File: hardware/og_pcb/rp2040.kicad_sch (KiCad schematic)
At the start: 29 parts, among them J11 Conn_02x02_Top_Bottom, J4 Micro_SD_Card_Det1, SW4 SW_Push_Shielded, SW5 SW_Push_Shielded, U12 RP2040, U3 W25Q128JVS, Y3 ABM8-272-T3

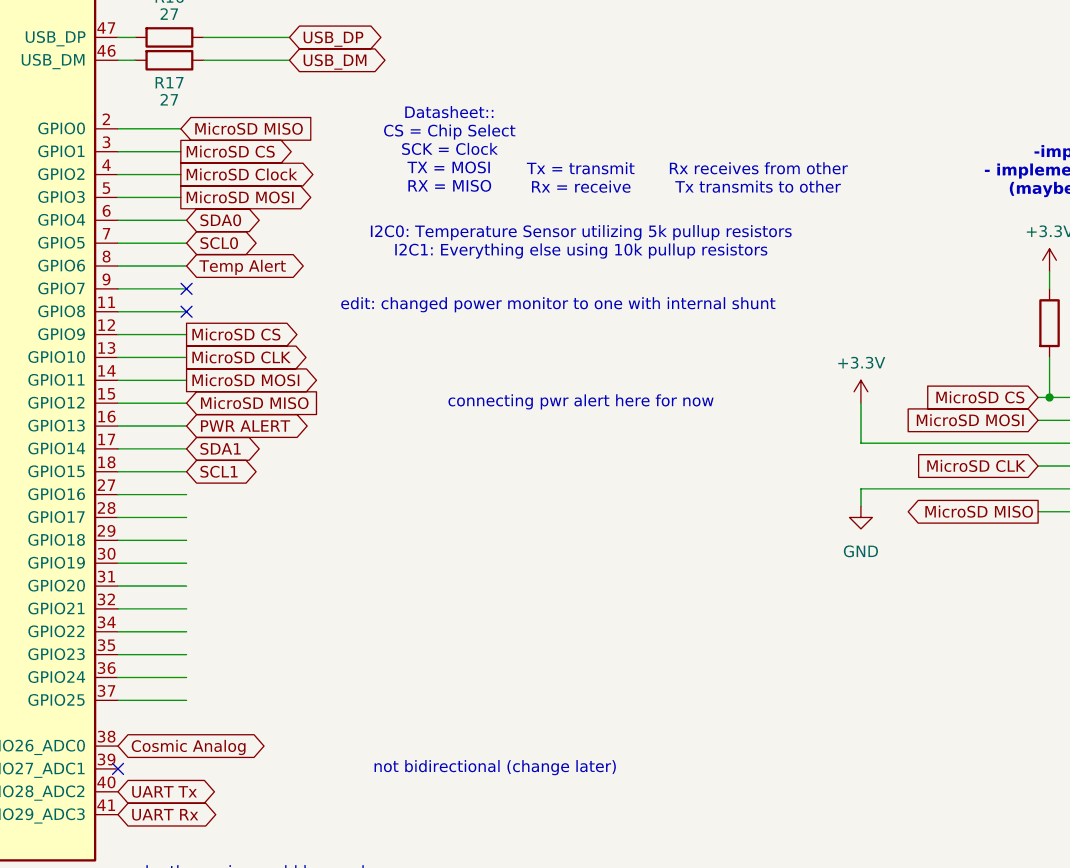
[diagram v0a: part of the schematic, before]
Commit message: new preliminary demo pcb
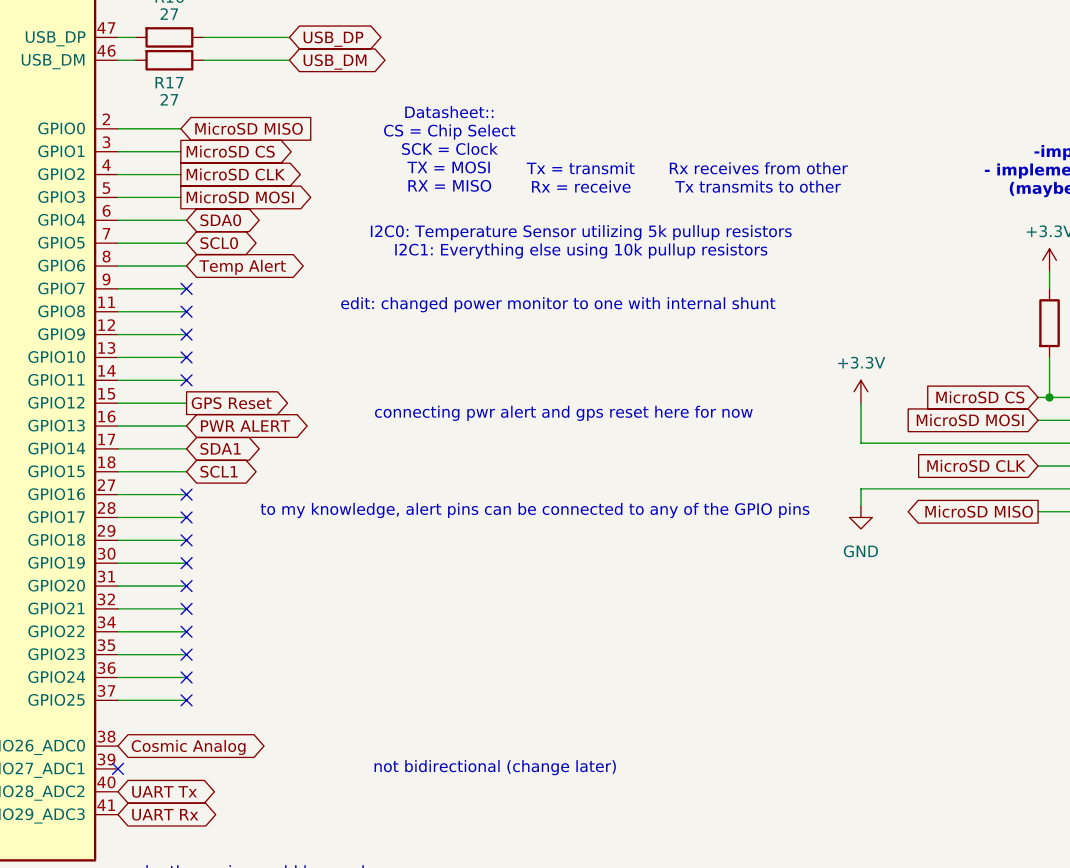
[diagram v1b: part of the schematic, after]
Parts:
- J4: footprint (none) -> 1my_footprints:microSD-503398-1892-1
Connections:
- net MicroSD Clock is gone; now on net MicroSD CLK: U12.4 (GPIO2)
- net MicroSD CLK: no longer U12.13 (GPIO10)
- net MicroSD CS: no longer U12.12 (GPIO9)
- net MicroSD MISO: no longer U12.15 (GPIO12)
- net MicroSD MOSI: no longer U12.14 (GPIO11)
- new net GPS Reset: U12.15 (GPIO12)
- no-connect marks 6 -> 19
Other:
- note added: "connecting pwr alert and gps reset here for now"
- note added: "to my knowledge, alert pins can be connected to any of the GPIO pins"
- note removed: "connecting pwr alert here for now"
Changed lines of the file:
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@@
 		)
 	)
+	(text "to my knowledge, alert pins can be connected to any of the GPIO pins"
+		(exclude_from_sim no)
+		(at 163.83 138.43 0)
+		(effects
+			(font
+				(size 1.27 1.27)
+			)
+		)
+	)
 	(text "Flash"
 		(exclude_from_sim no)
@@
 		)
 	)
-	(text "connecting pwr alert here for now"
+	(text "connecting pwr alert and gps reset here for now"
 		(exclude_from_sim no)
-		(at 168.91 126.365 0)
+		(at 167.005 127.635 0)
 		(effects
 			(font
@@
 	)
 	(no_connect
+		(at 125.095 154.305)
+	)
+	(no_connect
 		(at 227.33 146.05)
 	)
 	(no_connect
+		(at 125.095 149.225)
+	)
+	(no_connect
+		(at 125.095 159.385)
+	)
+	(no_connect
 		(at 125.095 116.205)
 	)
 	(no_connect
+		(at 125.095 146.685)
+	)
+	(no_connect
 		(at 125.095 113.665)
 	)
@@
 	)
 	(no_connect
+		(at 125.095 136.525)
+	)
+	(no_connect
+		(at 125.095 139.065)
+	)
+	(no_connect
+		(at 125.095 123.825)
+	)
+	(no_connect
 		(at 227.33 140.97)
 	)
 	(no_connect
+		(at 125.095 118.745)
+	)
+	(no_connect
+		(at 125.095 144.145)
+	)
+	(no_connect
+		(at 125.095 121.285)
+	)
+	(no_connect
+		(at 125.095 151.765)
+	)
+	(no_connect
 		(at 227.33 123.19)
 	)
+	(no_connect
+		(at 125.095 156.845)
+	)
+	(no_connect
+		(at 125.095 141.605)
+	)
 	(wire
 		(pts
@@
 		)
 	)
-	(global_label "MicroSD CS"
-		(shape output)
-		(at 125.095 118.745 0)
-		(fields_autoplaced yes)
-		(effects
-			(font
-				(size 1.27 1.27)
-			)
-			(justify left)
-		)
-		(property "Intersheetrefs" "${INTERSHEET_REFS}"
-			(at 139.0868 118.745 0)
-			(effects
-				(font
-					(size 1.27 1.27)
-				)
-				(justify left)
-				(hide yes)
-			)
-		)
-	)
 	(global_label "MicroSD MOSI"
 		(shape input)
@@
 		)
 	)
-	(global_label "MicroSD CLK"
-		(shape output)
-		(at 125.095 121.285 0)
-		(fields_autoplaced yes)
-		(effects
-			(font
-				(size 1.27 1.27)
-			)
-			(justify left)
-		)
-		(property "Intersheetrefs" "${INTERSHEET_REFS}"
-			(at 140.1754 121.285 0)
-			(effects
-				(font
-					(size 1.27 1.27)
-				)
-				(justify left)
-				(hide yes)
-			)
-		)
-	)
 	(global_label "SDA1"
 		(shape bidirectional)
@@
 		)
 	)
-	(global_label "Cosmic Analog"
-		(shape bidirectional)
-		(at 117.475 164.465 0)
+	(global_label "GPS Reset"
+		(shape output)
+		(at 125.095 126.365 0)
 		(fields_autoplaced yes)
 		(effects
@@
 		)
 		(property "Intersheetrefs" "${INTERSHEET_REFS}"
-			(at 135.7227 164.465 0)
+			(at 137.9983 126.365 0)
 			(effects
 				(font
@@
 		)
 	)
-	(global_label "MicroSD CS"
-		(shape input)
-		(at 219.71 125.73 180)
-		(fields_autoplaced yes)
-		(effects
-			(font
-				(size 1.27 1.27)
-			)
-			(justify right)
-		)
-		(property "Intersheetrefs" "${INTERSHEET_REFS}"
-			(at 205.7182 125.73 0)
-			(effects
-				(font
-					(size 1.27 1.27)
-				)
-				(justify right)
-				(hide yes)
-			)
-		)
-	)
-	(global_label "MicroSD MISO"
-		(shape input)
-		(at 125.095 126.365 0)
+	(global_label "MicroSD CLK"
+		(shape output)
+		(at 124.46 100.965 0)
 		(fields_autoplaced yes)
 		(effects
@@
 		)
 		(property "Intersheetrefs" "${INTERSHEET_REFS}"
-			(at 141.2035 126.365 0)
+			(at 139.5404 100.965 0)
 			(effects
 				(font
@@
 		)
 	)
-	(global_label "PWR ALERT"
+	(global_label "Cosmic Analog"
 		(shape bidirectional)
-		(at 125.095 128.905 0)
+		(at 117.475 164.465 0)
 		(fields_autoplaced yes)
 		(effects
 			(font
 				(size 1.27 1.27)
-				(thickness 0.1588)
 			)
 			(justify left)
 		)
 		(property "Intersheetrefs" "${INTERSHEET_REFS}"
-			(at 139.6538 128.905 0)
+			(at 135.7227 164.465 0)
 			(effects
 				(font
@@
 		)
 	)
-	(global_label "MicroSD CLK"
+	(global_label "MicroSD CS"
 		(shape input)
-		(at 219.71 133.35 180)
+		(at 219.71 125.73 180)
 		(fields_autoplaced yes)
 		(effects
@@
 		)
 		(property "Intersheetrefs" "${INTERSHEET_REFS}"
-			(at 204.6296 133.35 0)
+			(at 205.7182 125.73 0)
 			(effects
 				(font
@@
 		)
 	)
-	(global_label "UART Tx"
+	(global_label "PWR ALERT"
 		(shape bidirectional)
-		(at 117.475 169.545 0)
+		(at 125.095 128.905 0)
 		(fields_autoplaced yes)
 		(effects
 			(font
 				(size 1.27 1.27)
+				(thickness 0.1588)
 			)
 			(justify left)
 		)
 		(property "Intersheetrefs" "${INTERSHEET_REFS}"
-			(at 129.1915 169.545 0)
+			(at 139.6538 128.905 0)
 			(effects
 				(font
@@
 		)
 	)
-	(global_label "SCL0"
-		(shape bidirectional)
-		(at 125.095 108.585 0)
+	(global_label "MicroSD CLK"
+		(shape input)
+		(at 219.71 133.35 180)
 		(fields_autoplaced yes)
 		(effects
@@
 				(size 1.27 1.27)
 			)
-			(justify left)
+			(justify right)
 		)
 		(property "Intersheetrefs" "${INTERSHEET_REFS}"
-			(at 133.9086 108.585 0)
+			(at 204.6296 133.35 0)
 			(effects
 				(font
 					(size 1.27 1.27)
 				)
-				(justify left)
+				(justify right)
 				(hide yes)
 			)
 		)
 	)
-	(global_label "MicroSD MOSI"
-		(shape output)
-		(at 125.095 123.825 0)
+	(global_label "UART Tx"
+		(shape bidirectional)
+		(at 117.475 169.545 0)
 		(fields_autoplaced yes)
 		(effects
@@
 		)
 		(property "Intersheetrefs" "${INTERSHEET_REFS}"
-			(at 141.2035 123.825 0)
+			(at 129.1915 169.545 0)
 			(effects
 				(font
@@
 		)
 	)
-	(global_label "SDA0"
+	(global_label "SCL0"
 		(shape bidirectional)
-		(at 125.095 106.045 0)
+		(at 125.095 108.585 0)
 		(fields_autoplaced yes)
 		(effects
@@
 		)
 		(property "Intersheetrefs" "${INTERSHEET_REFS}"
-			(at 133.9691 106.045 0)
+			(at 133.9086 108.585 0)
 			(effects
 				(font
@@
 		)
 	)
-	(global_label "MicroSD Clock"
-		(shape output)
-		(at 124.46 100.965 0)
+	(global_label "SDA0"
+		(shape bidirectional)
+		(at 125.095 106.045 0)
 		(fields_autoplaced yes)
 		(effects
@@
 		)
 		(property "Intersheetrefs" "${INTERSHEET_REFS}"
-			(at 141.1732 100.965 0)
+			(at 133.9691 106.045 0)
 			(effects
 				(font
@@
 			)
 		)
-		(property "Footprint" ""
+		(property "Footprint" "1my_footprints:microSD-503398-1892-1"
 			(at 302.26 115.57 0)
 			(effects
